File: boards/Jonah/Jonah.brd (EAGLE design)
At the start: 54.6 x 25.4 mm, 10 parts

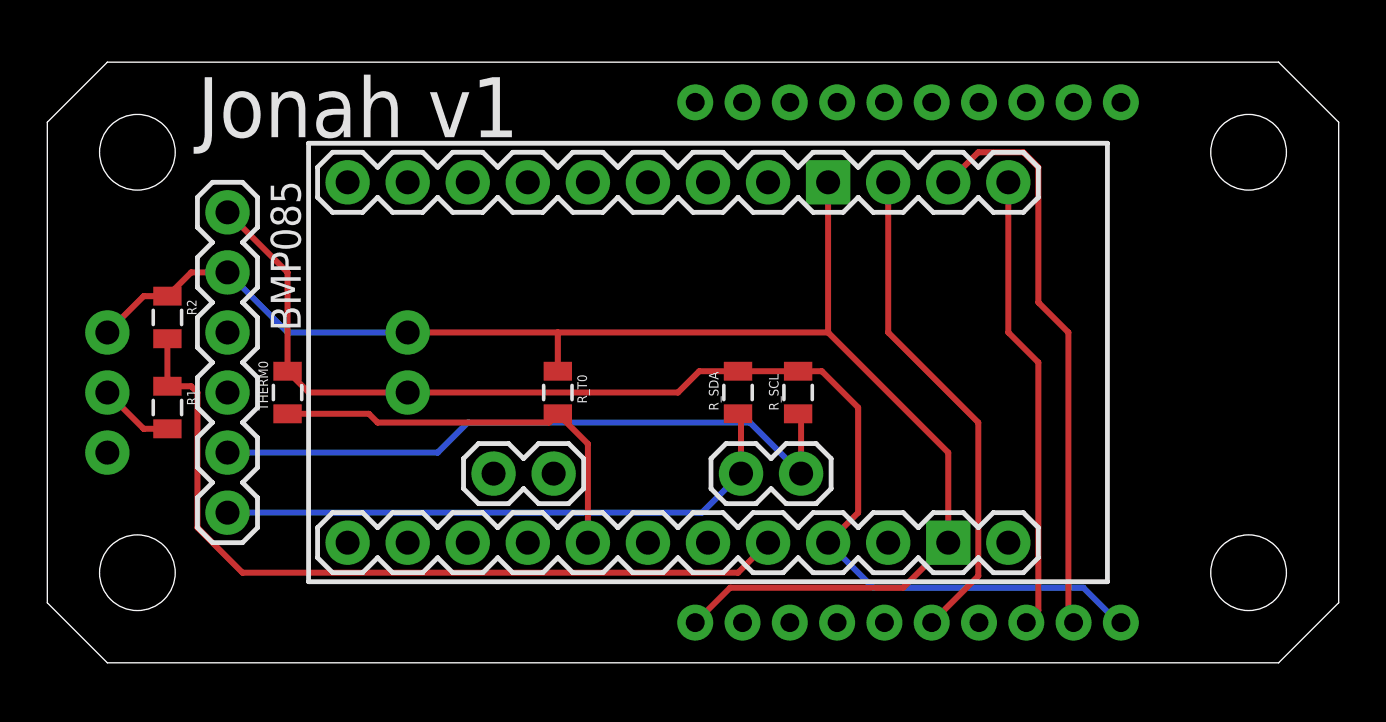
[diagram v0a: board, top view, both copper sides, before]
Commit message: First pass at Jonah board v2
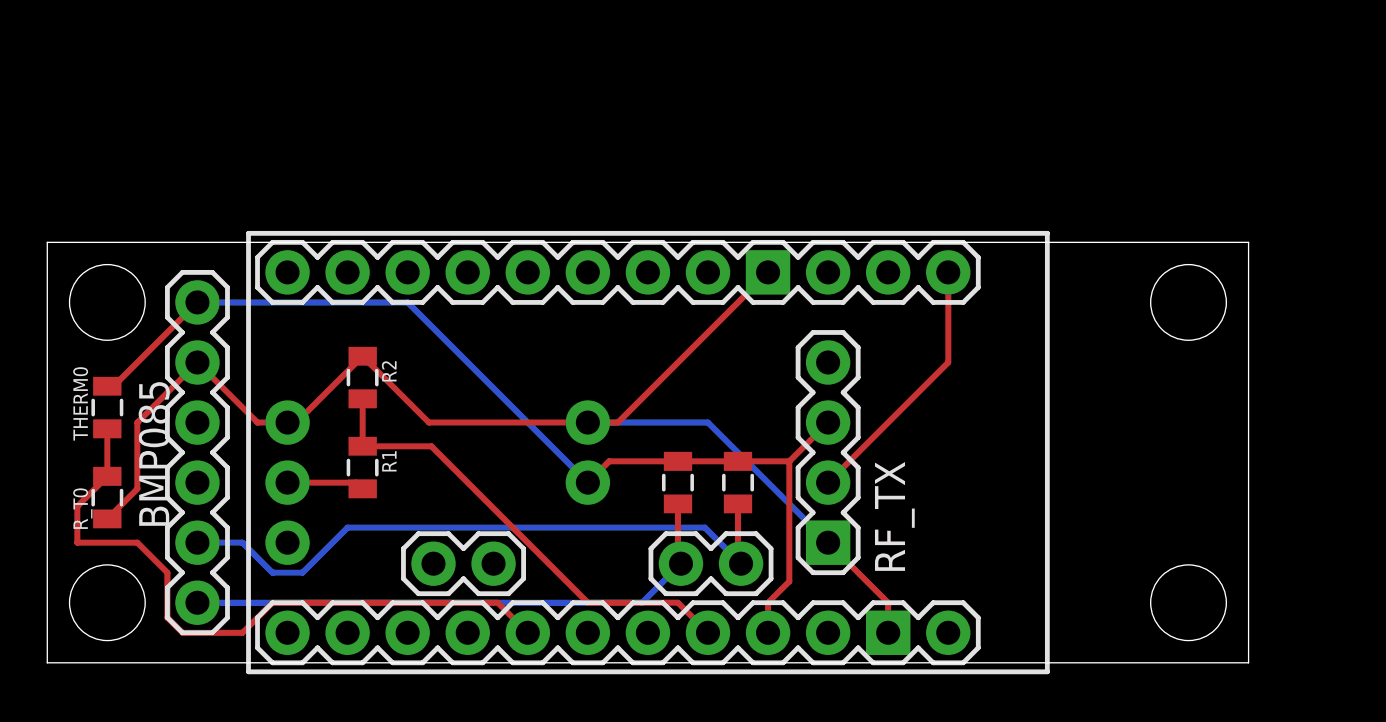
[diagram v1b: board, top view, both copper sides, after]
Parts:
- removed XBEE: XBEE-1B2, SparkFun-RF:XBEE-SILK
- added RF_TX: 434 MHz, SparkFun-Connectors:1X04
- moved R_T0 19.6 mm to (2.54, 6.99), turned to 90 degrees
- moved R2 8.64 mm to (13.3, 12.1)
- moved R1 8.64 mm to (13.3, 8.26)
- moved MAIN 8.52 mm to (12.7, 8.89)
- moved THERM0 7.65 mm to (2.54, 10.8)
- moved ARDUINO 4.58 mm to (24.1, 8.89)
- moved R_SCL 4.58 mm to (29.2, 7.62)
- moved R_SDA 4.58 mm to (26.7, 7.62)
- moved BMP085 4.02 mm to (6.35, 15.2)
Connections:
- removed net N$3: ARDUINO.TXO, XBEE.3
- removed net N$4: ARDUINO.RXI, XBEE.2
- net 3.3V: now also RF_TX.3; no longer XBEE.1
- net GND: now also RF_TX.1; no longer XBEE.10
- net N$1: now also ARDUINO.TXO, RF_TX.2; no longer ARDUINO.RST0, XBEE.5
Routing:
- net N$4: track 24.5 -> 0.00 mm
- net N$3: track 19.4 -> 0.00 mm
- net N$2: track 34.5 -> 19.9 mm
- net A0: track 17.7 -> 28.1 mm
- net N$1: track 21.0 -> 11.0 mm
- net 3.3V: track 53.3 -> 43.8 mm
- net GND: track 63.7 -> 55.5 mm
- net SDA: track 25.0 -> 23.7 mm
- net SCL: track 28.3 -> 27.5 mm
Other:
- board size 54.6 x 25.4 mm -> 50.8 x 17.8 mm
- board text added: "Jonah v2"
- board text removed: "Jonah v1"
